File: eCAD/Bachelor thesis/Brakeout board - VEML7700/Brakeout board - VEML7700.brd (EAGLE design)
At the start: 12.7 x 12.4 mm, 5 parts, among them IC1 VEML7700-TR

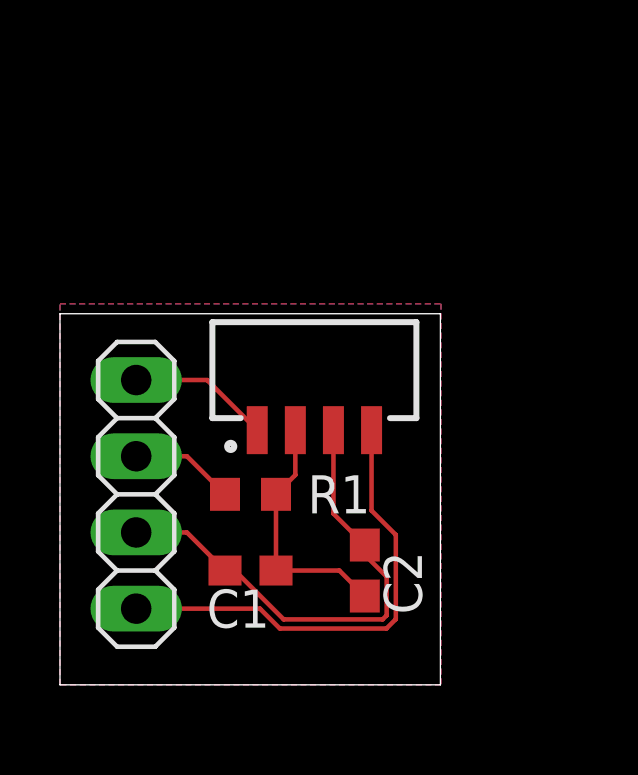
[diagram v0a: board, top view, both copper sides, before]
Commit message: Final touches
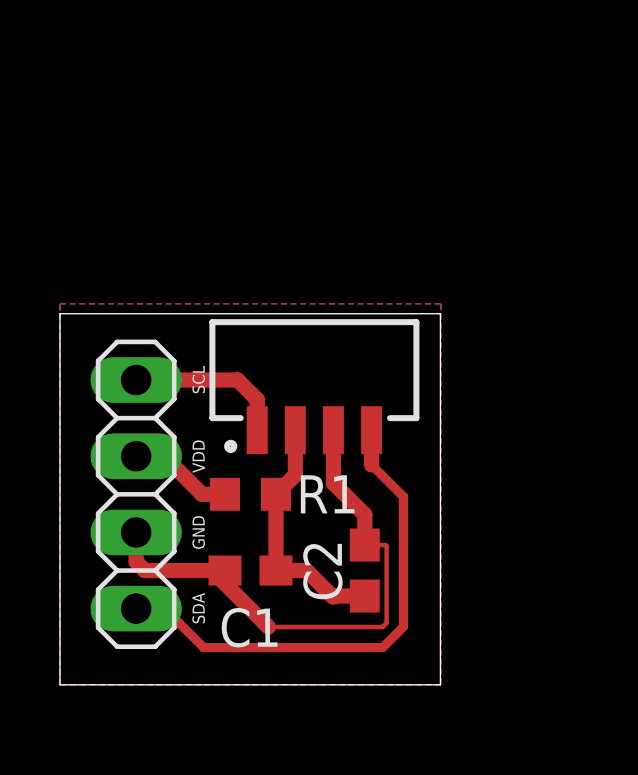
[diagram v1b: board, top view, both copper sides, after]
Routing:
- net GND: track 16.5 -> 18.3 mm
- net SDA: track 15.7 -> 16.7 mm
- net SCL: track 4.73 -> 5.32 mm
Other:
- board text added: "GND"
- board text added: "SCL"
- board text added: "SDA"
- board text added: "VDD"
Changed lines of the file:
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@@
 <setting verticaltext="up"/>
 </settings>
-<grid distance="50" unitdist="mil" unit="mil" style="lines" multiple="1" display="no" altdistance="5" altunitdist="mil" altunit="mil"/>
+<grid distance="10" unitdist="mil" unit="mil" style="lines" multiple="1" display="no" altdistance="5" altunitdist="mil" altunit="mil"/>
 <layers>
 <layer number="1" name="Top" color="4" fill="1" visible="yes" active="yes"/>
@@
 <wire x1="12.68" y1="12.37" x2="0" y2="12.37" width="0" layer="20"/>
 <wire x1="0" y1="12.37" x2="0" y2="0" width="0" layer="20"/>
+<text x="4.826" y="10.16" size="0.4064" layer="25" rot="R90" align="bottom-center">SCL</text>
+<text x="4.826" y="7.62" size="0.4064" layer="25" rot="R90" align="bottom-center">VDD</text>
+<text x="4.826" y="5.08" size="0.4064" layer="25" rot="R90" align="bottom-center">GND</text>
+<text x="4.826" y="2.54" size="0.4064" layer="25" rot="R90" align="bottom-center">SDA</text>
 </plain>
 <attributes>
@@
 </element>
 <element name="R1" library="rcl" library_urn="urn:adsk.eagle:library:334" package="R0603" package3d_urn="urn:adsk.eagle:package:23555/3" value="10R" x="6.35" y="6.35" smashed="yes">
-<attribute name="NAME" x="8.255" y="5.715" size="1.27" layer="25"/>
+<attribute name="NAME" x="7.874" y="6.35" size="1.27" layer="25" align="center-left"/>
 <attribute name="POPULARITY" value="70" x="6.35" y="6.35" size="1.778" layer="27" display="off"/>
 <attribute name="SPICEPREFIX" value="R" x="6.35" y="6.35" size="1.778" layer="27" display="off"/>
 </element>
 <element name="C1" library="rcl" library_urn="urn:adsk.eagle:library:334" package="C0603" package3d_urn="urn:adsk.eagle:package:23616/2" value="10u" x="6.35" y="3.81" smashed="yes" rot="R180">
-<attribute name="NAME" x="6.985" y="3.175" size="1.27" layer="25" rot="R180"/>
+<attribute name="NAME" x="6.35" y="2.54" size="1.27" layer="25" align="top-center"/>
 <attribute name="POPULARITY" value="73" x="6.35" y="3.81" size="1.778" layer="27" rot="R180" display="off"/>
 <attribute name="SPICEPREFIX" value="C" x="6.35" y="3.81" size="1.778" layer="27" rot="R180" display="off"/>
 </element>
 <element name="C2" library="rcl" library_urn="urn:adsk.eagle:library:334" package="C0603" package3d_urn="urn:adsk.eagle:package:23616/2" value="100n" x="10.16" y="3.81" smashed="yes" rot="R90">
-<attribute name="NAME" x="10.795" y="4.445" size="1.27" layer="25" rot="R270"/>
+<attribute name="NAME" x="8.128" y="3.81" size="1.27" layer="25" rot="R90" align="top-center"/>
 <attribute name="POPULARITY" value="73" x="10.16" y="3.81" size="1.778" layer="27" rot="R90" display="off"/>
 <attribute name="SPICEPREFIX" value="C" x="10.16" y="3.81" size="1.778" layer="27" rot="R90" display="off"/>
@@
 <contactref element="C2" pad="2"/>
 <contactref element="VEML_BRAKEOUT" pad="2"/>
-<wire x1="10.16" y1="4.66" x2="9.115" y2="5.705" width="0.1524" layer="1"/>
-<wire x1="9.115" y1="5.705" x2="9.115" y2="8.49" width="0.1524" layer="1"/>
-<wire x1="2.54" y1="5.08" x2="4.23" y2="5.08" width="0.1524" layer="1"/>
-<wire x1="4.23" y1="5.08" x2="5.5" y2="3.81" width="0.1524" layer="1"/>
-<wire x1="10.7546875" y1="2.1814" x2="10.8886" y2="2.3153125" width="0.1524" layer="1"/>
-<wire x1="10.8886" y1="2.3153125" x2="10.8886" y2="3.6046875" width="0.1524" layer="1"/>
-<wire x1="5.5" y1="3.81" x2="5.8267125" y2="3.81" width="0.1524" layer="1"/>
-<wire x1="10.16" y1="4.3332875" x2="10.16" y2="4.66" width="0.1524" layer="1"/>
-<wire x1="10.8886" y1="3.6046875" x2="10.16" y2="4.3332875" width="0.1524" layer="1"/>
-<wire x1="5.8267125" y1="3.81" x2="7.4553125" y2="2.1814" width="0.1524" layer="1"/>
-<wire x1="7.4553125" y1="2.1814" x2="10.7546875" y2="2.1814" width="0.1524" layer="1"/>
+<wire x1="10.16" y1="4.66" x2="10.16" y2="5.676" width="0.508" layer="1"/>
+<wire x1="10.16" y1="5.676" x2="9.115" y2="6.721" width="0.508" layer="1"/>
+<wire x1="9.115" y1="6.721" x2="9.115" y2="8.49" width="0.508" layer="1"/>
+<wire x1="2.833" y1="3.81" x2="5.5" y2="3.81" width="0.508" layer="1"/>
+<wire x1="2.833" y1="3.81" x2="2.54" y2="4.103" width="0.508" layer="1"/>
+<wire x1="2.54" y1="5.08" x2="2.54" y2="4.103" width="0.508" layer="1"/>
+<wire x1="10.7546875" y1="1.9274" x2="10.8886" y2="2.0613125" width="0.1524" layer="1"/>
+<wire x1="10.8886" y1="2.0613125" x2="10.8886" y2="4.6206875" width="0.1524" layer="1"/>
+<wire x1="10.16" y1="4.66" x2="10.8492875" y2="4.66" width="0.1524" layer="1"/>
+<wire x1="10.8886" y1="4.6206875" x2="10.8492875" y2="4.66" width="0.1524" layer="1"/>
+<wire x1="5.5" y1="3.81" x2="5.28235625" y2="3.59235625" width="0.1524" layer="1"/>
+<wire x1="6.9473125" y1="1.9274" x2="5.28235625" y2="3.59235625" width="0.508" layer="1"/>
+<wire x1="6.9473125" y1="1.9274" x2="10.7546875" y2="1.9274" width="0.1524" layer="1"/>
 <polygon width="0.1524" layer="1">
 <vertex x="0" y="0"/>
@@
 <contactref element="VEML_BRAKEOUT" pad="3"/>
 <contactref element="R1" pad="1"/>
-<wire x1="2.54" y1="7.62" x2="4.23" y2="7.62" width="0.1524" layer="1"/>
-<wire x1="4.23" y1="7.62" x2="5.5" y2="6.35" width="0.1524" layer="1"/>
+<wire x1="2.54" y1="7.62" x2="3.468" y2="7.62" width="0.508" layer="1"/>
+<wire x1="4.738" y1="6.35" x2="5.5" y2="6.35" width="0.508" layer="1"/>
+<wire x1="4.738" y1="6.35" x2="3.468" y2="7.62" width="0.508" layer="1"/>
 </signal>
 <signal name="N$2">
@@
 <contactref element="C1" pad="1"/>
 <contactref element="C2" pad="1"/>
-<wire x1="7.2" y1="6.35" x2="7.845" y2="6.995" width="0.1524" layer="1"/>
-<wire x1="7.845" y1="6.995" x2="7.845" y2="8.49" width="0.1524" layer="1"/>
-<wire x1="7.2" y1="3.81" x2="7.2" y2="6.35" width="0.1524" layer="1"/>
-<wire x1="7.2" y1="3.81" x2="9.31" y2="3.81" width="0.1524" layer="1"/>
-<wire x1="9.31" y1="3.81" x2="10.16" y2="2.96" width="0.1524" layer="1"/>
+<wire x1="7.2" y1="6.35" x2="7.845" y2="6.995" width="0.508" layer="1"/>
+<wire x1="7.845" y1="6.995" x2="7.845" y2="8.49" width="0.508" layer="1"/>
+<wire x1="7.2" y1="3.81" x2="7.2" y2="6.35" width="0.508" layer="1"/>
+<wire x1="9.105" y1="2.921" x2="8.216" y2="3.81" width="0.508" layer="1"/>
+<wire x1="7.2" y1="3.81" x2="8.216" y2="3.81" width="0.508" layer="1"/>
+<wire x1="9.144" y1="2.96" x2="10.16" y2="2.96" width="0.508" layer="1"/>
+<wire x1="9.144" y1="2.96" x2="9.105" y2="2.921" width="0.3048" layer="1"/>
 </signal>
 <signal name="SCL">
 <contactref element="VEML_BRAKEOUT" pad="4"/>
 <contactref element="IC1" pad="1"/>
-<wire x1="2.54" y1="10.16" x2="4.905" y2="10.16" width="0.1524" layer="1"/>
-<wire x1="4.905" y1="10.16" x2="6.575" y2="8.49" width="0.1524" layer="1"/>
+<wire x1="2.54" y1="10.16" x2="5.921" y2="10.16" width="0.508" layer="1"/>
+<wire x1="6.575" y1="9.506" x2="6.575" y2="8.49" width="0.508" layer="1"/>
+<wire x1="6.575" y1="9.506" x2="5.921" y2="10.16" width="0.508" layer="1"/>
 </signal>
 <signal name="SDA">
 <contactref element="VEML_BRAKEOUT" pad="1"/>
 <contactref element="IC1" pad="4"/>
-<wire x1="7.32905625" y1="1.8766" x2="10.88094375" y2="1.8766" width="0.1524" layer="1"/>
-<wire x1="10.88094375" y1="1.8766" x2="11.1934" y2="2.18905625" width="0.1524" layer="1"/>
-<wire x1="6.66565625" y1="2.54" x2="7.32905625" y2="1.8766" width="0.1524" layer="1"/>
-<wire x1="2.54" y1="2.54" x2="6.66565625" y2="2.54" width="0.1524" layer="1"/>
-<wire x1="11.1934" y1="2.18905625" x2="11.1934" y2="4.9998875" width="0.1524" layer="1"/>
-<wire x1="11.1934" y1="4.9998875" x2="10.385" y2="5.8082875" width="0.1524" layer="1"/>
-<wire x1="10.385" y1="5.8082875" x2="10.385" y2="8.49" width="0.1524" layer="1"/>
+<wire x1="4.78905625" y1="1.2416" x2="10.75394375" y2="1.2416" width="0.3048" layer="1"/>
+<wire x1="10.75394375" y1="1.2416" x2="11.4474" y2="1.93505625" width="0.3048" layer="1"/>
+<wire x1="3.49065625" y1="2.54" x2="4.78905625" y2="1.2416" width="0.3048" layer="1"/>
+<wire x1="2.54" y1="2.54" x2="3.49065625" y2="2.54" width="0.508" layer="1"/>
+<wire x1="11.4474" y1="1.93505625" x2="11.4474" y2="6.2698875" width="0.3048" layer="1"/>
+<wire x1="11.4474" y1="6.2698875" x2="10.385" y2="7.3322875" width="0.3048" layer="1"/>
+<wire x1="10.385" y1="7.3322875" x2="10.385" y2="8.49" width="0.508" layer="1"/>
 </signal>
 </signals>

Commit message: Production files
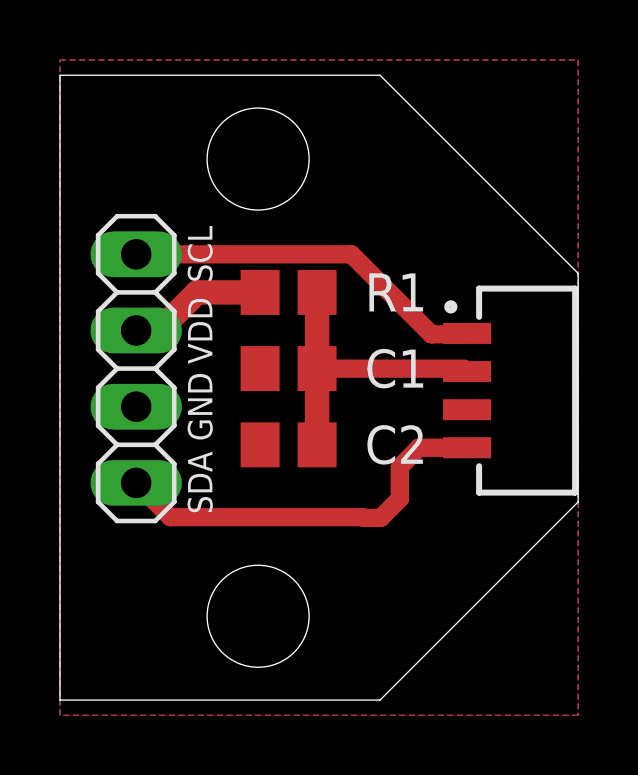
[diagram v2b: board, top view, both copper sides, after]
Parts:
- C1, C2: device rcl:C0603 -> rcl:C0805
- R1: device rcl:R0603 -> rcl:R0805
- moved IC1 9.88 mm to (14.0, 13.2), turned to 270 degrees
- moved C1 6.85 mm to (7.62, 10.5)
- moved R1 6.85 mm to (7.62, 13.1)
- moved C2 4.90 mm to (7.62, 8.00), turned to 180 degrees
- moved VEML_BRAKEOUT 4.19 mm to (2.54, 10.5)
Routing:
- net GND: track 18.3 -> 0.00 mm
- net SCL: track 5.32 -> 12.1 mm
- net SDA: track 16.7 -> 13.2 mm
- net N$2: track 8.29 -> 10.1 mm
- net VDD: track 3.49 -> 4.66 mm
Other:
- board size 12.7 x 12.4 mm -> 17.3 x 20.8 mm
- board text added: "VEML7700 brakeout board"
